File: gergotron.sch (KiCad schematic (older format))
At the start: 8 parts, among them P1 Power, P2 Analog, P3 Digital, P4 Digital, P5 CONN_01X01, P6 CONN_01X01, P7 CONN_01X01, P8 CONN_01X01

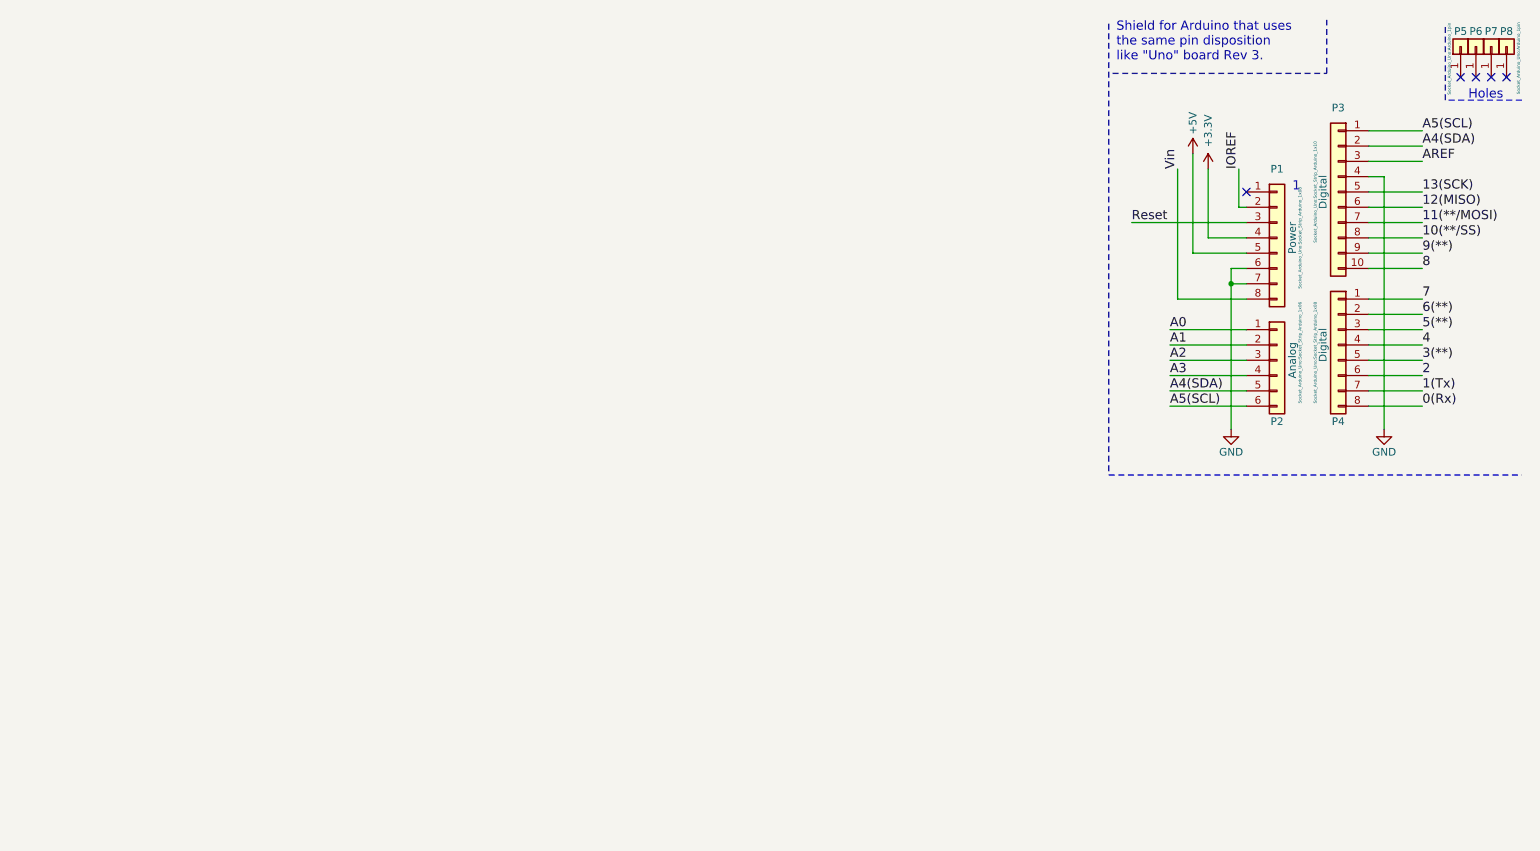
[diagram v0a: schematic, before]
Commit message: ps/2 done
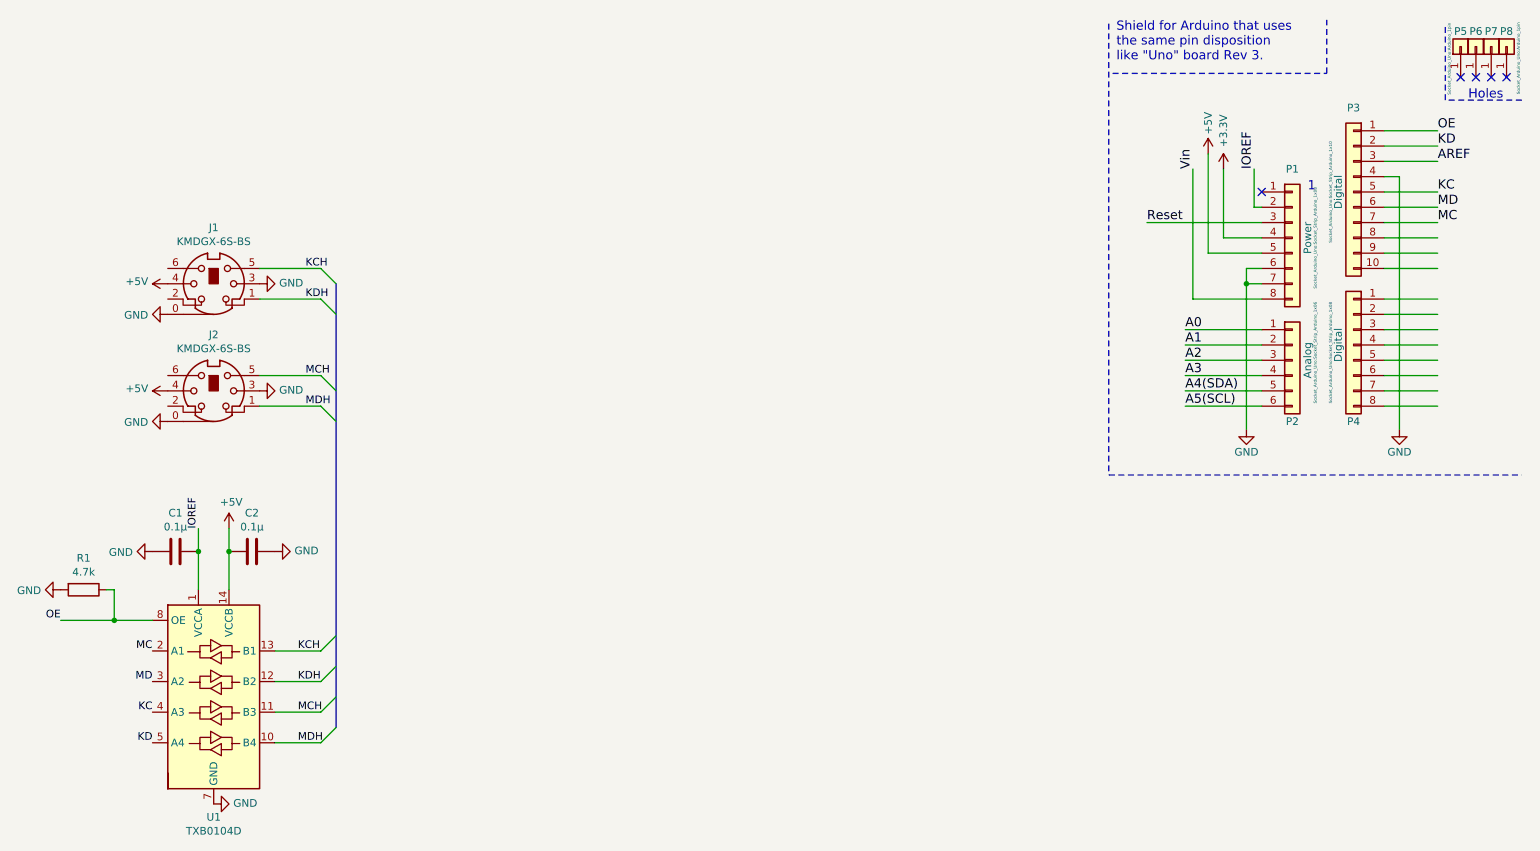
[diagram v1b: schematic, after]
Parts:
- added C1, C2: 0.1μ, Capacitor_SMD:C_0603_1608Metric, symbol Device:C
- added J1, J2: KMDGX-6S-BS, gergotron:kmdgx-6s-bs, symbol kmdgx-6s-bs:KMDGX-6S-BS
- added R1: 4.7k, Resistor_SMD:R_0603_1608Metric, symbol Device:R
- added U1: TXB0104D, Package_SO:SOIC-14_3.9x8.7mm_P1.27mm, symbol Logic_LevelTranslator:TXB0104D
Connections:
- net labels added: KC, KCH, KD, KDH, MC, MCH, MD, MDH, OE
- net labels removed: 0(Rx), 1(Tx), 10(**/SS), 11(**/MOSI), 12(MISO), 13(SCK), 2, 3(**), 4, 5(**), 6(**), 7, 8, 9(**)
- wire segments 38 -> 54
